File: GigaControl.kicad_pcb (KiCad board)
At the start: 6 copper layers, 34.4 x 20 mm, 51 parts, among them J1 Conn_02x10_Odd_Even, J2 Conn_02x10_Odd_Even, J3 Conn_02x10_Odd_Even, U1 LSM6DS3TR-C, U2 SIT3051, U3 REF3033AIDBZR, U4 PESD4USB5U-TTSX, U5 PESD4USB5U-TTSX, U6 STM32F405RGT6, U7 PESD4USB5U-TTSX, U8 PESD4USB5U-TTSX, Y1 SX2M8.000M20F30TNN

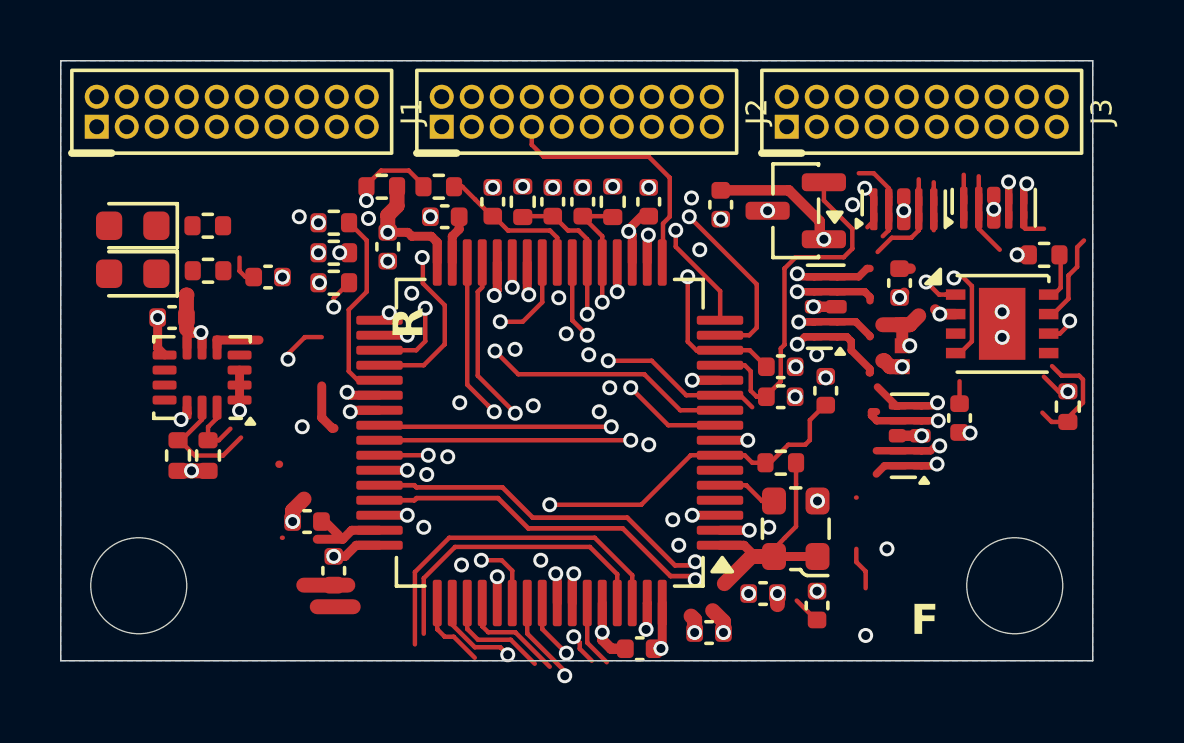
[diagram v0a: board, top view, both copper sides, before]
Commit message: pre-full-route
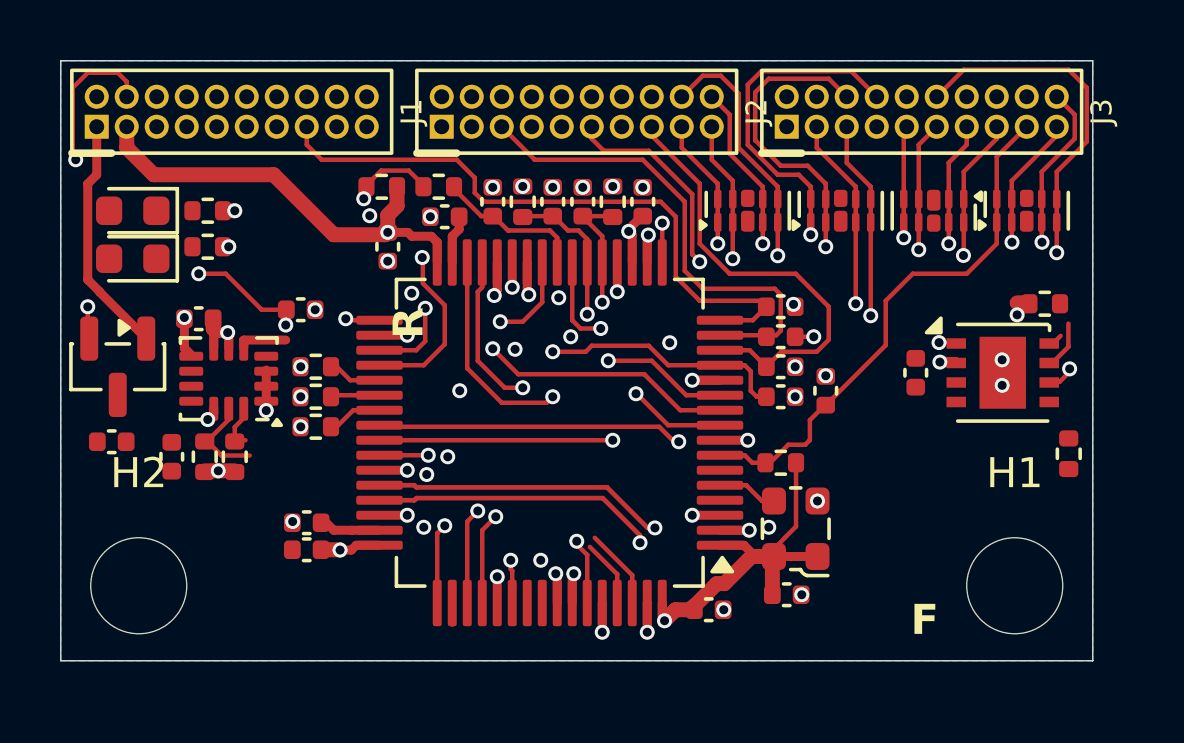
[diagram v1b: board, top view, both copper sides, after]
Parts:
- removed JP3: VSel, X3.0CH-Library:SolderJumper-3-0.5-Small
- H1, H2: value MountingHole_3.2mm_M3 -> MountingHole; footprint MountingHole:MountingHole_3.2mm_M3 -> MountingHole:MountingHole_3.2mm_M3_DIN965
- moved H1 29.2 mm to (169.2, 103.0)
- moved H2 29.2 mm to (140.0, 103.0)
- moved U3 23.2 mm to (139.3, 95.7), turned to -90 degrees
- moved C5 21.8 mm to (139.1, 98.2), turned to 0 degrees
- moved C1 18.8 mm to (141.1, 98.7), turned to -90 degrees
- moved C27 9.04 mm to (161.4, 94.7), turned to 0 degrees
- moved U8 7.54 mm to (166.5, 90.5), turned to -90 degrees
- moved C28 7.02 mm to (161.4, 93.7), turned to 0 degrees
- moved R15 4.84 mm to (145.9, 97.7)
- moved R16 4.84 mm to (145.9, 96.7)
- moved R17 4.84 mm to (145.9, 95.7)
- moved U4 4.12 mm to (160.3, 90.5), turned to 90 degrees
- moved C3 3.04 mm to (165.9, 95.9)
- moved C17 2.64 mm to (159.0, 103.8), turned to 0 degrees
- moved U7 2.10 mm to (163.4, 90.5)
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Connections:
- J2 pad 17: SPI1-MOSI -> SPI1-NSS
- J2 pad 18: USBD- -> SPI1-MOSI
- J2 pad 19: SPI1-MISO-ADC2 -> SPI1-SCK-ADC
- J2 pad 20: USBD+ -> SPI1-MISO-ADC2
- J3 pad 1: GND -> USBD+
- J3 pad 12: HALL3 IN -> SERVO
- J3 pad 13: SERVO -> HALL3 IN
- J3 pad 14: TEMPMOTOR IN -> IN-CANL
- J3 pad 15: NRST -> TEMPMOTOR IN
- J3 pad 16: I2C2 SDA/USART3 RX -> IN-CANH
- J3 pad 17: I2C2 SCL/USART3 TX -> NRST
- J3 pad 18: SWDIO -> GND
- J3 pad 19: SWCLK -> ESP-TX
- J3 pad 2: SPI1-SCK-ADC -> USBD-
- J3 pad 20: GND -> ESP-RX
- J3 pad 3: ESP-TX -> SWDIO
- J3 pad 4: SPI1-NSS -> GND
- J3 pad 5: ESP-RX -> SWCLK
- J3 pad 6: IN-CANH -> I2C2 SDA/USART3 RX
- J3 pad 7: HALL-VOLTAGE -> GND
- J3 pad 8: IN-CANL -> I2C2 SCL/USART3 TX
- U4 pad 1: SPI1-MOSI -> SPI1-NSS
- U4 pad 10: SPI1-MOSI -> SPI1-NSS
- U4 pad 2: SPI1-MISO-ADC2 -> SPI1-SCK-ADC
- U4 pad 4: SPI1-SCK-ADC -> SPI1-MISO-ADC2
- U4 pad 5: SPI1-NSS -> SPI1-MOSI
- U4 pad 6: SPI1-NSS -> SPI1-MOSI
- U4 pad 7: SPI1-SCK-ADC -> SPI1-MISO-ADC2
- U4 pad 9: SPI1-MISO-ADC2 -> SPI1-SCK-ADC
- U5 pad 2: SERVO -> ESP-TX
- U5 pad 4: I2C2 SDA/USART3 RX -> ESP-RX
- U5 pad 5: I2C2 SCL/USART3 TX -> SERVO
- U5 pad 6: I2C2 SCL/USART3 TX -> SERVO
- U5 pad 7: I2C2 SDA/USART3 RX -> ESP-RX
- U5 pad 9: SERVO -> ESP-TX
- U7 pad 1: SWDIO -> I2C2 SCL/USART3 TX
- U7 pad 10: SWDIO -> I2C2 SCL/USART3 TX
- U7 pad 2: SWCLK -> I2C2 SDA/USART3 RX
- U7 pad 4: ESP-TX -> SWDIO
- U7 pad 5: ESP-RX -> SWCLK
- U7 pad 6: ESP-RX -> SWCLK
- U7 pad 7: ESP-TX -> SWDIO
- U7 pad 9: SWCLK -> I2C2 SDA/USART3 RX
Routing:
- net SERVO: track 4.93 -> 34.8 mm, vias 0 -> 2
- net ESP-RX: track 5.40 -> 31.4 mm, vias 0 -> 2
- net ESP-TX: track 6.97 -> 30.0 mm, vias 0 -> 2
- net SWCLK: track 5.57 -> 27.3 mm, vias 0 -> 2
- net HALL3 IN: track 10.5 -> 29.0 mm
- net SWDIO: track 8.70 -> 26.6 mm
- net HALL2 IN: track 11.1 -> 27.6 mm
- net USBD-: track 18.0 -> 33.7 mm
- net HALL1 IN: track 11.3 -> 27.0 mm
- net USBD+: track 18.0 -> 33.7 mm
- net IN V: track 18.0 -> 32.3 mm, vias 1 -> 4
- net +3.3REF: track 12.0 -> 25.9 mm, vias 0 -> 2
- net LED FAULT: track 14.3 -> 0.88 mm, vias 2 -> 1
- net POWER STAGE LOCKOUT: track 5.25 -> 18.2 mm
- net TEMPMOTOR IN: track 16.7 -> 28.9 mm
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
